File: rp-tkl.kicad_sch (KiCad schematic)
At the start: 5 parts

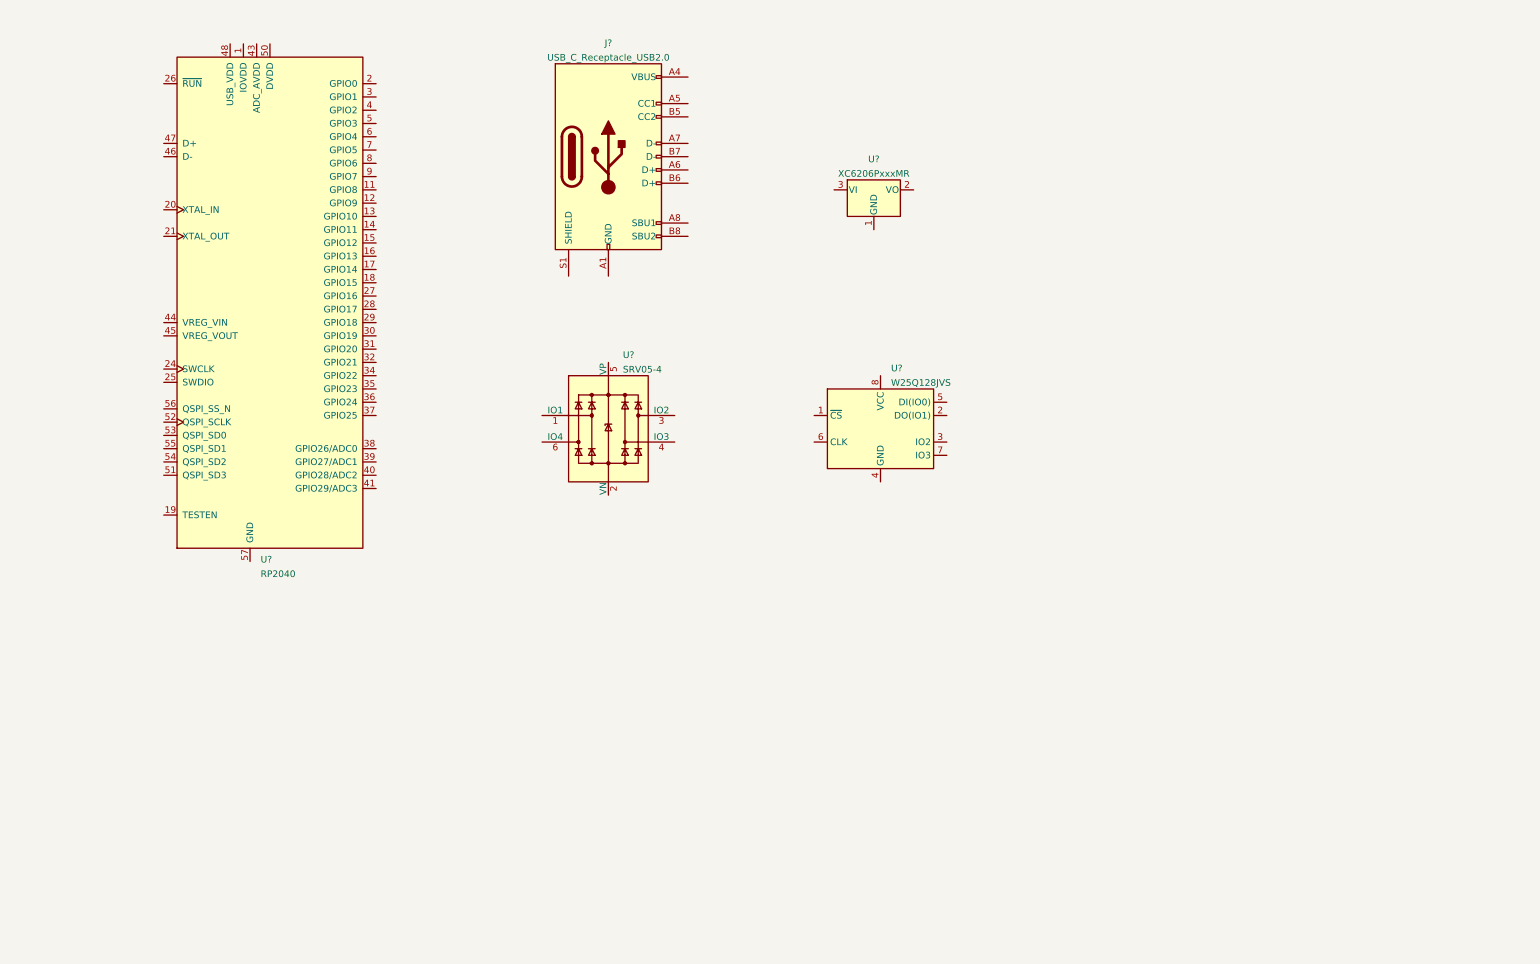
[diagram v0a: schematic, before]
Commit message: Finished most of preliminary schematic
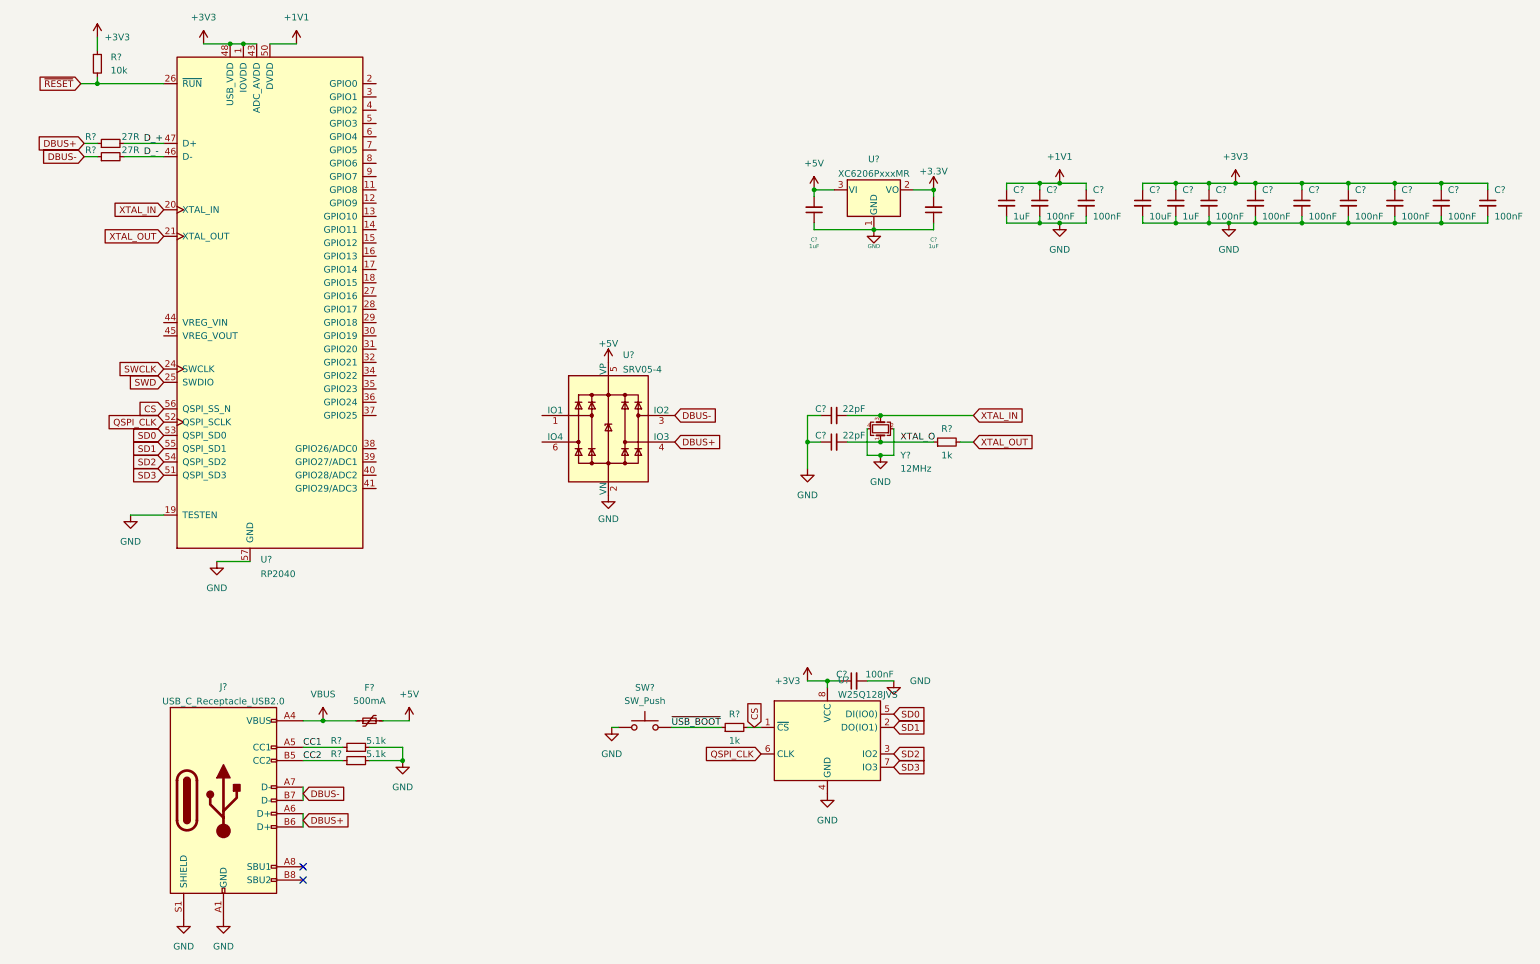
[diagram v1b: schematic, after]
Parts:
- added C?: 10uF, Capacitor_SMD:C_0402_1005Metric, symbol Device:C_Small
- added C? (x10): 100nF, Capacitor_SMD:C_0402_1005Metric, symbol Device:C_Small
- added C? (x4): 1uF, Capacitor_SMD:C_0402_1005Metric, symbol Device:C_Small
- added C? (x2): 22pF, Capacitor_SMD:C_0402_1005Metric, symbol Device:C_Small
- added F?: 500mA, Fuse:Fuse_1206_3216Metric, symbol Device:Polyfuse_Small
- added R? (x2): 1k, Resistor_SMD:R_0402_1005Metric, symbol Device:R_Small
- added R? (x2): 27R, Resistor_SMD:R_0603_1608Metric, symbol Device:R_Small
- added R? (x2): 5.1k, Resistor_SMD:R_0402_1005Metric, symbol Device:R_Small
- added R?: 10k, Resistor_SMD:R_0402_1005Metric, symbol Device:R_Small
- added SW?: SW_Push, Connector_PinSocket_2.54mm:PinSocket_1x02_P2.54mm_Vertical, symbol Switch:SW_Push
- added Y?: 12MHz, Crystal:Crystal_SMD_3225-4Pin_3.2x2.5mm, symbol Device:Crystal_GND24_Small
- J?: footprint (none) -> Connector_USB:USB_C_Receptacle_HRO_TYPE-C-31-M-12
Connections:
- net IOVDD is gone; now on net +3V3: U?.1 (IOVDD), U?.10 (IOVDD), U?.22 (IOVDD), U?.33 (IOVDD), U?.42 (IOVDD), U?.49 (IOVDD)
- net GND: now reaches U?.2 (VN)
- net GND: now also J?.A1 (GND), J?.A12 (GND), J?.B1 (GND), J?.B12 (GND), J?.S1 (SHIELD), U?.1 (GND), U?.19 (TESTEN), U?.4 (GND), U?.57 (GND), C?.1, C?.1, C?.1, C?.1, C?.2, C?.2, C?.2, C?.2, C?.2, C?.2, C?.2, C?.2, C?.2, C?.2, C?.2, C?.2, C?.2, R?.2, R?.2, SW?.1, Y?.2, Y?.4
- net DBUS-: now reaches U?.3 (IO2)
- net DBUS-: now also J?.A7 (D-), J?.B7 (D-), R?.1
- net DBUS+: now reaches U?.4 (IO3)
- net DBUS+: now also J?.A6 (D+), J?.B6 (D+), R?.1
- net +5V: now reaches U?.5 (VP)
- net +5V: now also U?.3 (VI), C?.2, F?.2
- net +3V3: now reaches U?.2 (VO)
- net +3V3: now also U?.43 (ADC_AVDD), U?.48 (USB_VDD), U?.8 (VCC), C?.1, C?.1, C?.1, C?.1, C?.1, C?.1, C?.1, C?.1, C?.1, C?.1, C?.2, R?.1
- net XTAL_IN: now reaches U?.20 (XTAL_IN)
- net XTAL_IN: now also C?.2, Y?.3
- net XTAL_OUT: now reaches U?.21 (XTAL_OUT)
- net XTAL_OUT: now also R?.2
- net SWCLK: now reaches U?.24 (SWCLK)
- net SWD: now reaches U?.25 (SWDIO)
- net ~{RESET}: now reaches U?.26 (~{RUN})
- net ~{RESET}: now also R?.2
- net D_-: now reaches U?.46 (D-)
- net D_-: now also R?.2
- net D_+: now reaches U?.47 (D+)
- net D_+: now also R?.2
- net SD3: now reaches U?.51 (QSPI_SD3)
- net SD3: now also U?.7 (IO3)
- net QSPI_CLK: now reaches U?.52 (QSPI_SCLK)
- net QSPI_CLK: now also U?.6 (CLK)
- net SD0: now reaches U?.53 (QSPI_SD0)
- net SD0: now also U?.5 (DI(IO0))
- net SD2: now reaches U?.54 (QSPI_SD2)
- net SD2: now also U?.3 (IO2)
- net SD1: now reaches U?.55 (QSPI_SD1)
- net SD1: now also U?.2 (DO(IO1))
- net CS: now reaches U?.56 (QSPI_SS_N)
- net CS: now also U?.1 (~{CS}), R?.2
- net VBUS: now reaches J?.A4 (VBUS), J?.A9 (VBUS), J?.B4 (VBUS), J?.B9 (VBUS)
- net VBUS: now also F?.1
- net CC1: now reaches J?.A5 (CC1)
- net CC1: now also R?.1
- net CC2: now reaches J?.B5 (CC2)
- net CC2: now also R?.1
- net DVDD renamed +1V1
- net +1V1: now also C?.1, C?.1, C?.1
- new net XTAL_O: C?.2, R?.1, Y?.1
- new net ~{USB_BOOT}: R?.1, SW?.2
- no-connect marks 0 -> 2
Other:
- moved on the sheet: J?, U?
